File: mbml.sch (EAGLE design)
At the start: 30 parts, among them K1 G5SB, Q1 2N2222, U1 LINEAR_REG_5V, U2 PHOTOCOUPLER, X1 43160-1102, X10 CON-2B2B-XH-A(LF)(SN), X2 CON-2, X3 CON-2B2B-XH-A(LF)(SN), X4 CON-2B2B-XH-A(LF)(SN), X5 CON-2B2B-XH-A(LF)(SN), X6 CON-2B2B-XH-A(LF)(SN), X7 CON-2B2B-XH-A(LF)(SN), X8 CON-2B2B-XH-A(LF)(SN), X9 CON-2B2B-XH-A(LF)(SN)

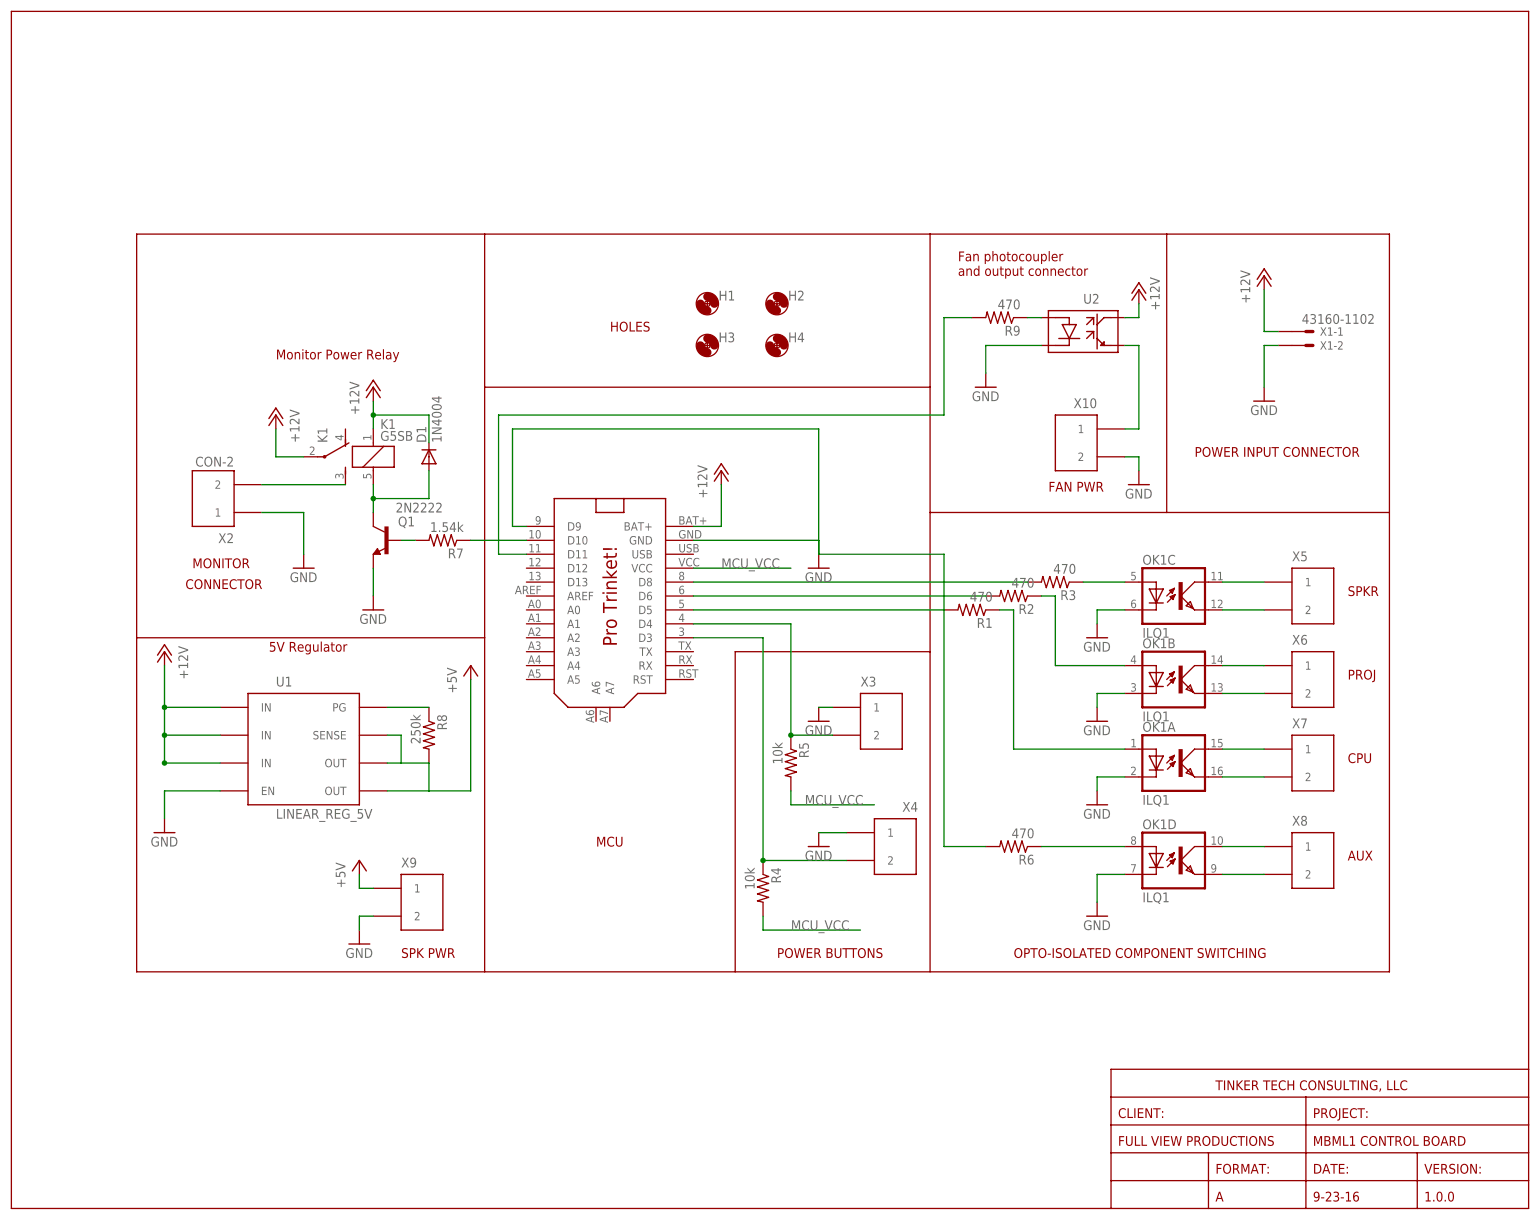
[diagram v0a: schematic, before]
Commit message: Starting major overhaul
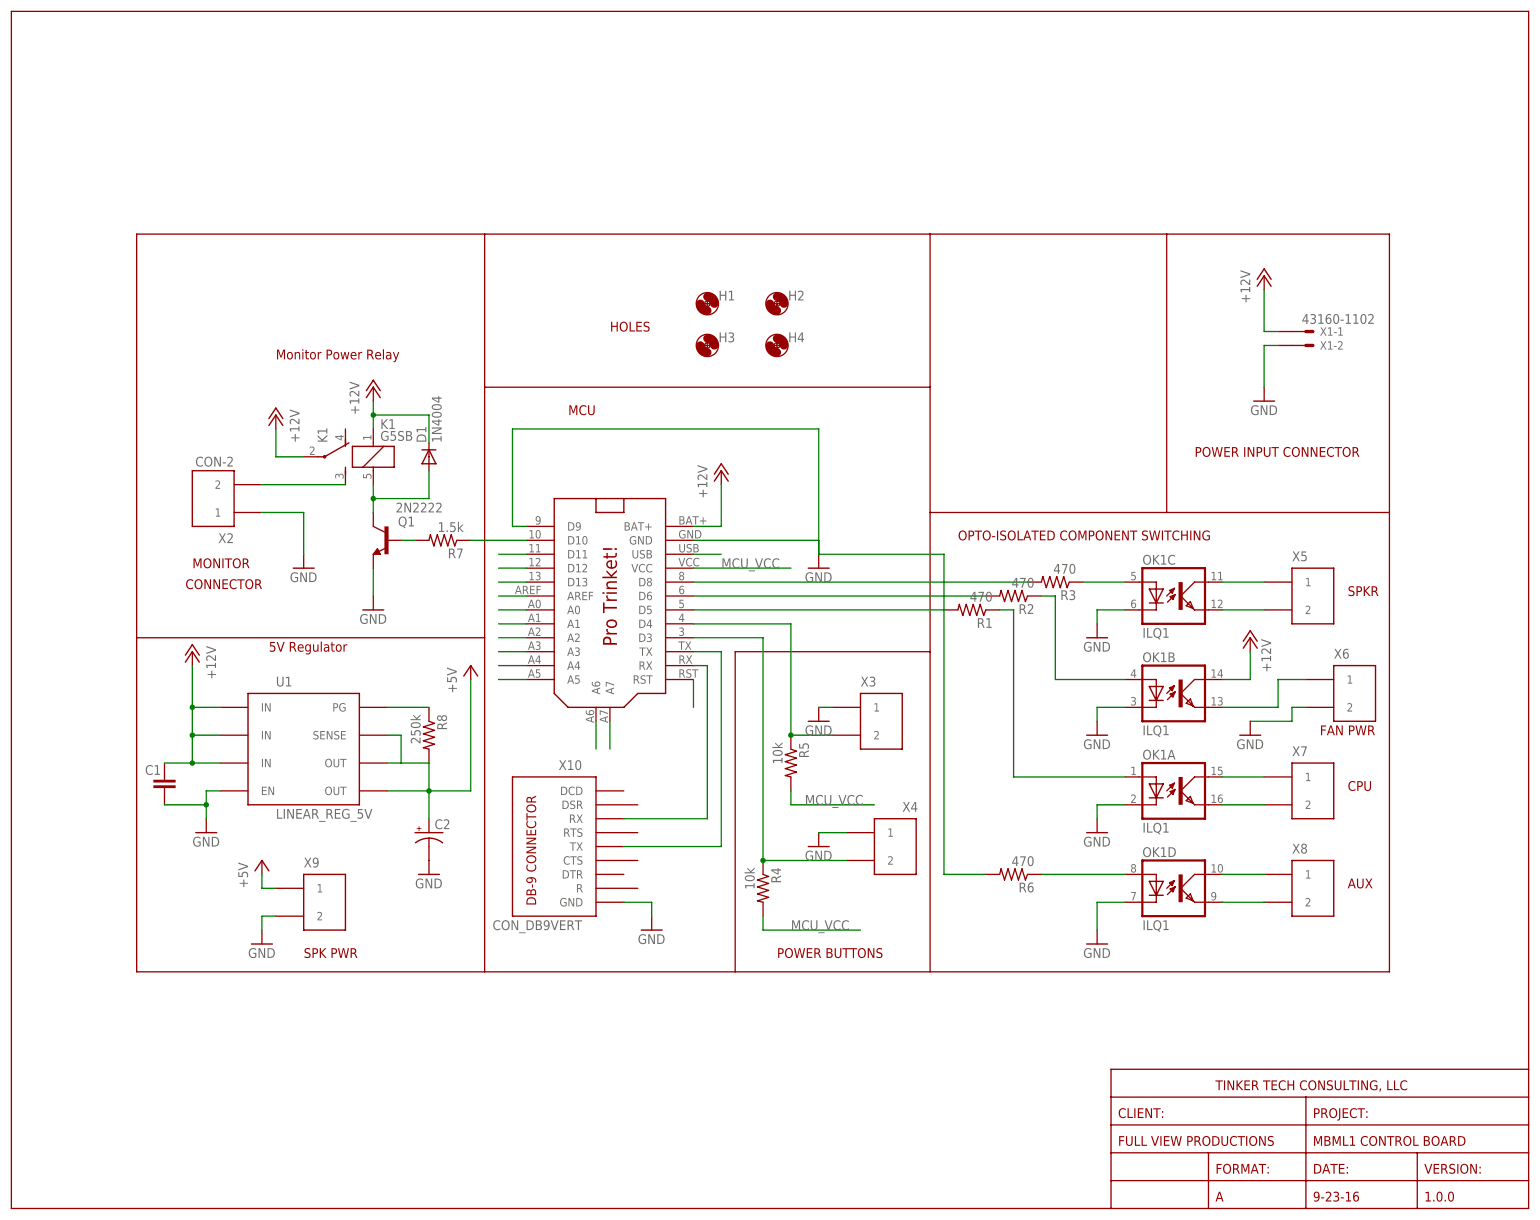
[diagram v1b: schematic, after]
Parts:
- removed R9: 470, resistor:R-US_0204/5
- removed U2: PHOTOCOUPLER, TinkerTech:PHOTOCOUPLER
- added C1: (no value), SparkFun-Passives:CAPPTH
- added C2: (no value), TinkerTech:CAP_POL
- R7: value 1.54k -> 1.5k
- X10: value CON-2B2B-XH-A(LF)(SN) -> CON_DB9VERT; device FVP:CON-2B2B-XH-A(LF)(SN) -> TinkerTech:CON_DB9VERT
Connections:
- net N$1 renamed D3
- net N$10 renamed D8
- net N$18 renamed D9
- net N$2 renamed D4
- net N$3 renamed TRANS_COLLECTOR
- net N$35 renamed D10
- net N$4 renamed D5
- net N$5 renamed TRANS_BASE
- net N$9 renamed D6
- removed net N$13: OK1B.COL, X6.1
- removed net N$46: R9.1, U2.P$1
- removed net N$47: R9.2, U$1.D11
- removed net N$49: U2.P$3, X10.1
- new net A0: U$1.A0
- new net A1: U$1.A1
- new net A2: U$1.A2
- new net A3: U$1.A3
- new net A4: U$1.A4
- new net A5: U$1.A5
- new net A6: U$1.A6
- new net A7: U$1.A7
- new net AREF: U$1.AREF
- new net D11: U$1.D11
- new net D12: U$1.D12
- new net D13: U$1.D13
- new net RST: U$1.RST
- new net RX: U$1.RX, X10.RX
- new net TX: U$1.TX, X10.TX
- new net USB: U$1.USB
- net +12V: now also C1.1, OK1B.COL; no longer U2.P$4
- net +5V: now also C2.+
- net GND: now also C1.2, C2.-, X10.GND, X6.2; no longer U2.P$2, X10.2
- net N$14: now also X6.1; no longer X6.2
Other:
- note removed: "Fan photocoupler and output connector"
- note removed: "PROJ"
- moved on the sheet: OK1A, OK1B, OK1D, R6, X6, X7, X8, X9

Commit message: Ready for production
Hopefully…
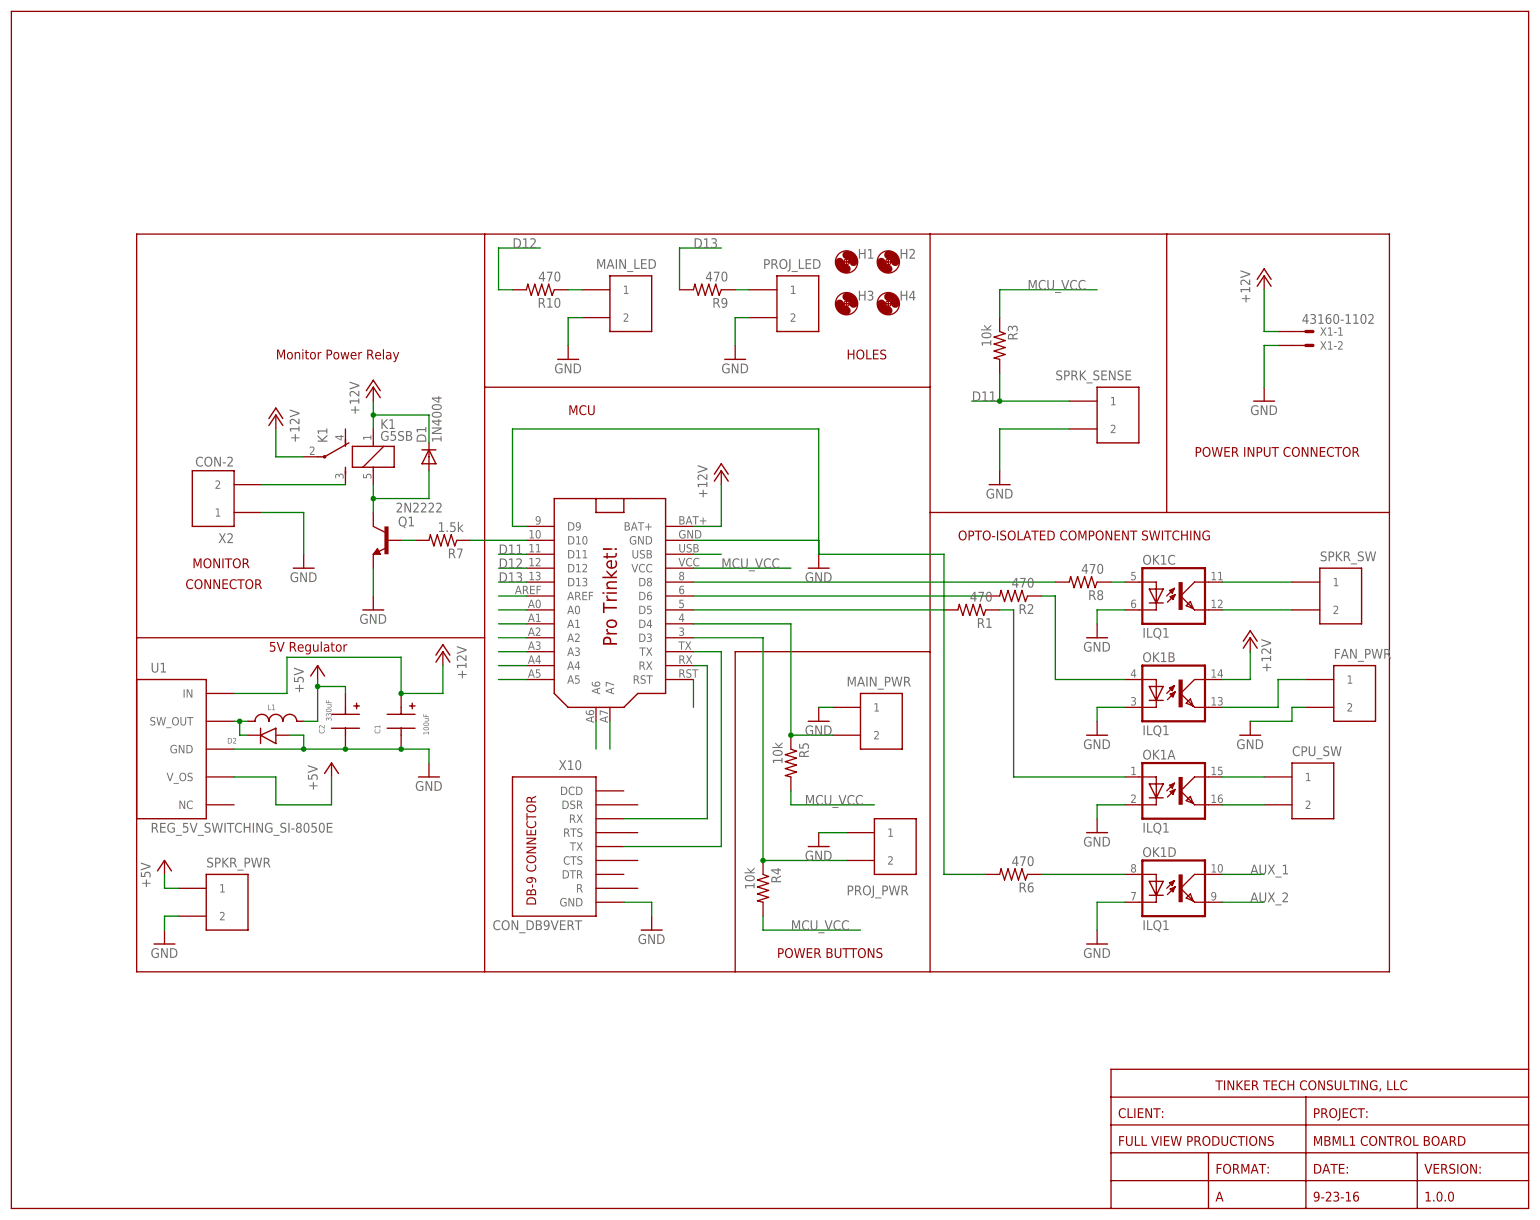
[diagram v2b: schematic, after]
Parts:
- removed X5, X8, X9: CON-2B2B-XH-A(LF)(SN), FVP:CON-2B2B-XH-A(LF)(SN)
- added D2: (no value), TinkerTech:DIODE
- added L1: (no value), TinkerTech:INDUCTORRADIAL_8.5-DIA_5-SPACE
- added MAIN_LED, PROJ_LED, SPKR_PWR, SPKR_SW, SPRK_SENSE: CON-2B2B-XH-A(LF)(SN), FVP:CON-2B2B-XH-A(LF)(SN)
- added R10, R9: 470, resistor:R-US_0204/5
- C1: value (none) -> 100uF; device SparkFun-Passives:CAPPTH -> TinkerTech:CAP_POL6.3-DIA_2.5-SPACE
- C2: value (none) -> 330uF; device TinkerTech:CAP_POL -> TinkerTech:CAP_POL10-DIA_5-SPACE
- R3: value 470 -> 10k
- R8: value 250k -> 470
- U1: value LINEAR_REG_5V -> REG_5V_SWITCHING_SI-8050E; device TinkerTech:LINEAR_REG_5V -> TinkerTech:REG_5V_SWITCHING_SI-8050E
- renumbered X3 to MAIN_PWR, X4 to PROJ_PWR, X6 to FAN_PWR, X7 to CPU_SW
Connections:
- removed net D8: R3.2, U$1.D8
- removed net N$12: OK1C.EMIT, X5.2
- removed net N$19: OK1D.COL, X8.1
- removed net N$20: OK1D.EMIT, X8.2
- removed net N$48: R8.1, U1.PG
- new net AUX_1: OK1D.COL
- new net AUX_2: OK1D.EMIT
- new net N$1: D2.-, L1.P$1, U1.SW_OUT
- new net N$2: OK1C.A, R8.1
- new net N$3: R8.2, U$1.D8
- new net N$4: OK1C.COL, SPKR_SW.1
- new net N$5: OK1C.EMIT, SPKR_SW.2
- net +12V: now also C1.+, U1.IN; no longer C1.1, U1.IN@1, U1.IN@2, U1.IN@3
- net +5V: now also L1.P$2, SPKR_PWR.1, U1.V_OS; no longer R8.2, U1.OUT@1, U1.OUT@2, U1.SENSE, X9.1
- net D11: now also R3.2, SPRK_SENSE.1
- net D12: now also R10.2
- net D13: now also R9.2
- net GND: now also C1.-, D2.+, MAIN_LED.2, PROJ_LED.2, SPKR_PWR.2, SPRK_SENSE.2, U1.GND; no longer C1.2, U1.EN, X9.2
- net MCU_VCC: now also R3.1
- net N$11: now also MAIN_LED.1, R10.1; no longer OK1C.COL, X5.1
- net N$6: now also PROJ_LED.1, R9.1; no longer OK1C.A, R3.1
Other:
- note removed: "AUX"
- note removed: "CPU"
- note removed: "FAN PWR"
- note removed: "SPK PWR"
- note removed: "SPKR"
- moved on the sheet: H1, H2, H3, H4, R3, R8

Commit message: Version 2.1, DRC OK
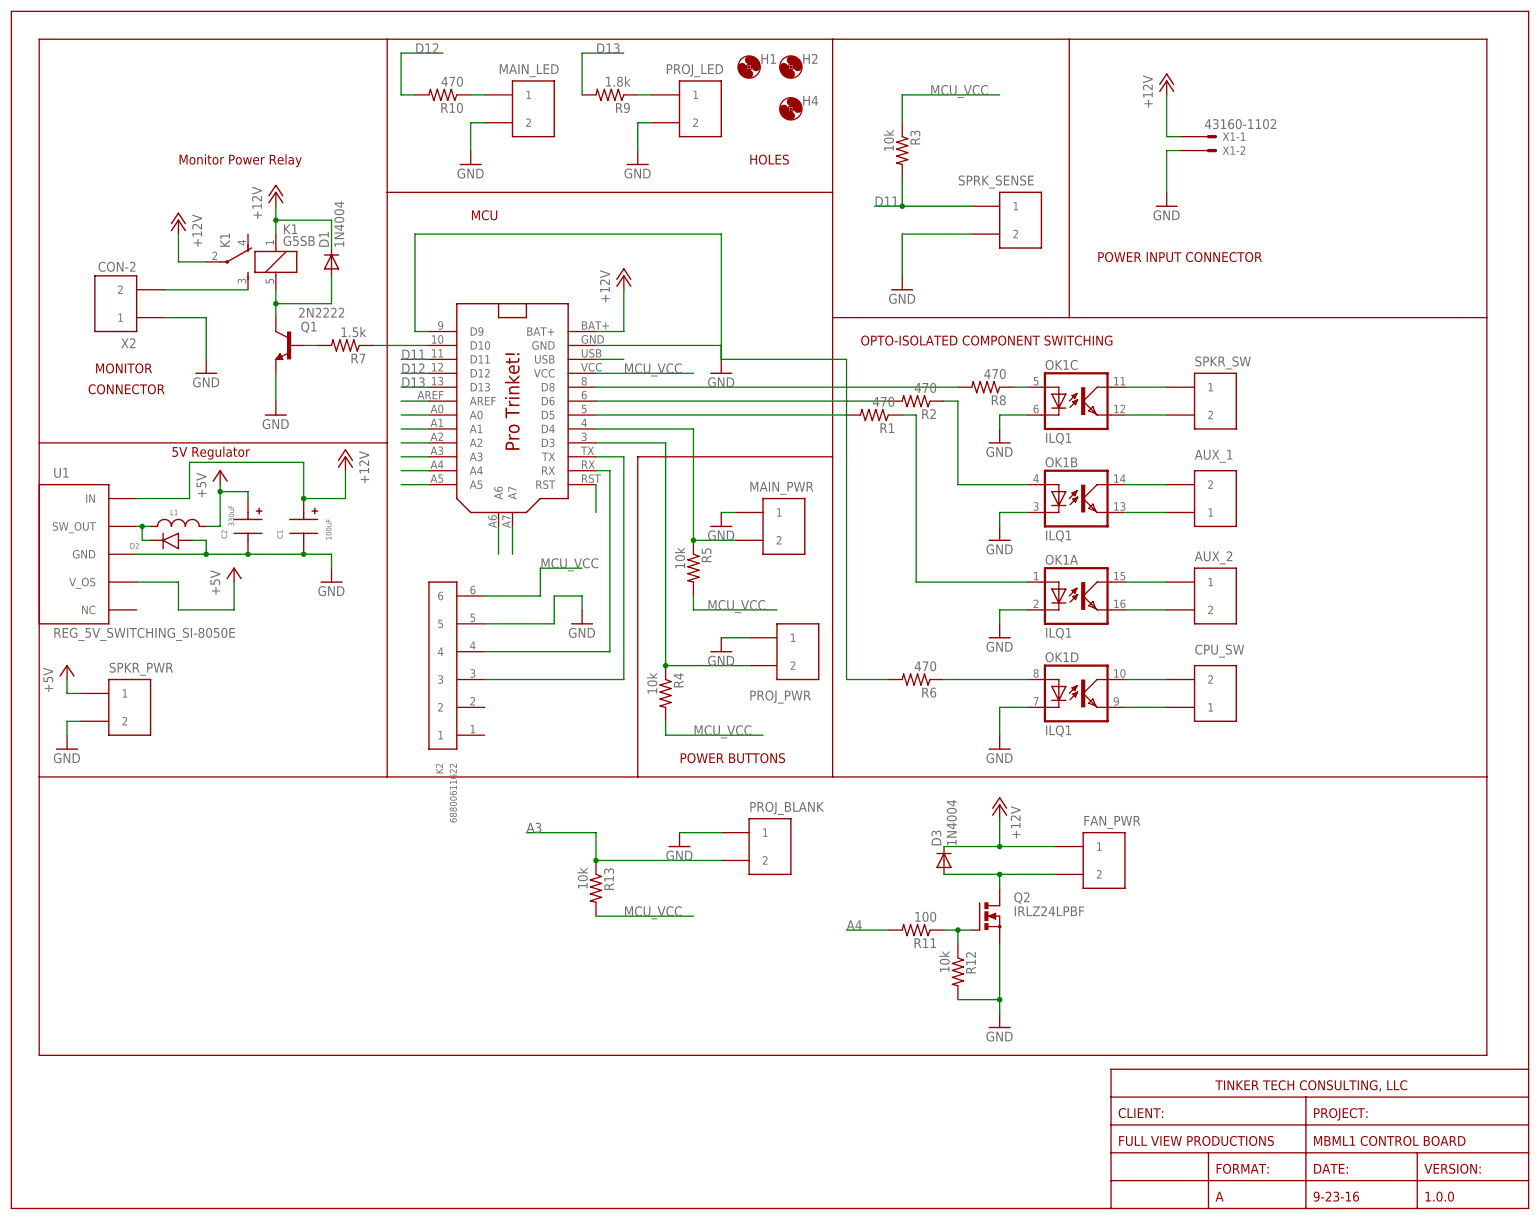
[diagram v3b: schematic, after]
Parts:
- removed H3: MOUNT-HOLE3.0, holes:MOUNT-HOLE3.0
- removed X10: CON_DB9VERT, TinkerTech:CON_DB9VERT
- added AUX_1, AUX_2, PROJ_BLANK: CON-2B2B-XH-A(LF)(SN), FVP:CON-2B2B-XH-A(LF)(SN)
- added D3: 1N4004, diode:1N4004
- added K2: 68800611622, Wurth_Wire_to_Board_Connectors_rev15d:68800611622
- added Q2: IRLZ24LPBF, transistor-power:PMOSFET_N
- added R11: 100, resistor:R-US_0204/5
- added R12, R13: 10k, resistor:R-US_0204/5
- R9: value 470 -> 1.8k
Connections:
- removed net AUX_1: OK1D.COL
- removed net AUX_2: OK1D.EMIT
- new net N$10: Q2.G, R11.1, R12.1
- new net N$12: AUX_1.2, OK1B.COL
- new net N$13: AUX_1.1, OK1B.EMIT
- new net N$18: CPU_SW.1, OK1D.EMIT
- new net N$9: D3.A, FAN_PWR.2, Q2.D
- net +12V: now also D3.C, FAN_PWR.1; no longer OK1B.COL
- net A3: now also PROJ_BLANK.2, R13.1
- net A4: now also R11.2
- net GND: now also K2.5, PROJ_BLANK.1, Q2.S, R12.2; no longer FAN_PWR.2, X10.GND
- net MCU_VCC: now also K2.6, R13.2
- net N$14: now also CPU_SW.2, OK1D.COL; no longer FAN_PWR.1, OK1B.EMIT
- net N$15: now also AUX_2.1; no longer CPU_SW.1
- net N$16: now also AUX_2.2; no longer CPU_SW.2
- net RX: now also K2.4; no longer X10.RX
- net TX: now also K2.3; no longer X10.TX
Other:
- moved on the sheet: C1, C2, CPU_SW, D1, D2, FAN_PWR, H1, H2, H4, K1, L1, MAIN_LED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
